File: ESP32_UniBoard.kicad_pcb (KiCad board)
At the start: 2 copper layers, 32 x 43.8 mm, 32 parts, among them J1 USB_C_Receptacle_USB2.0, J2 Conn_01x06_Socket, J3 Hirose DF40C, SW1 SW_Push, SW2 SW_Push, U1 ESP32-S3-WROOM-1, U2 SPX3819M5-L-3-3, U3 USBLC6-2SC6

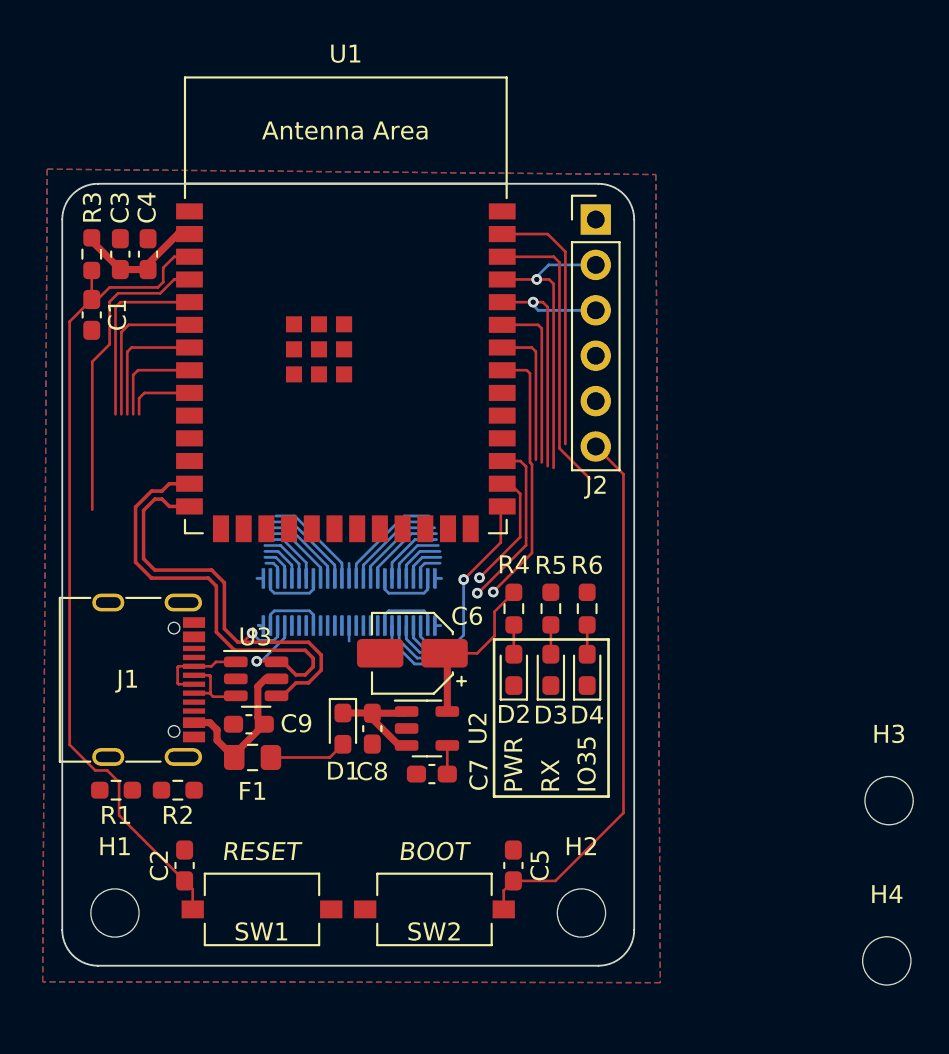
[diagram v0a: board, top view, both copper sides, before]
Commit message: PCB rework
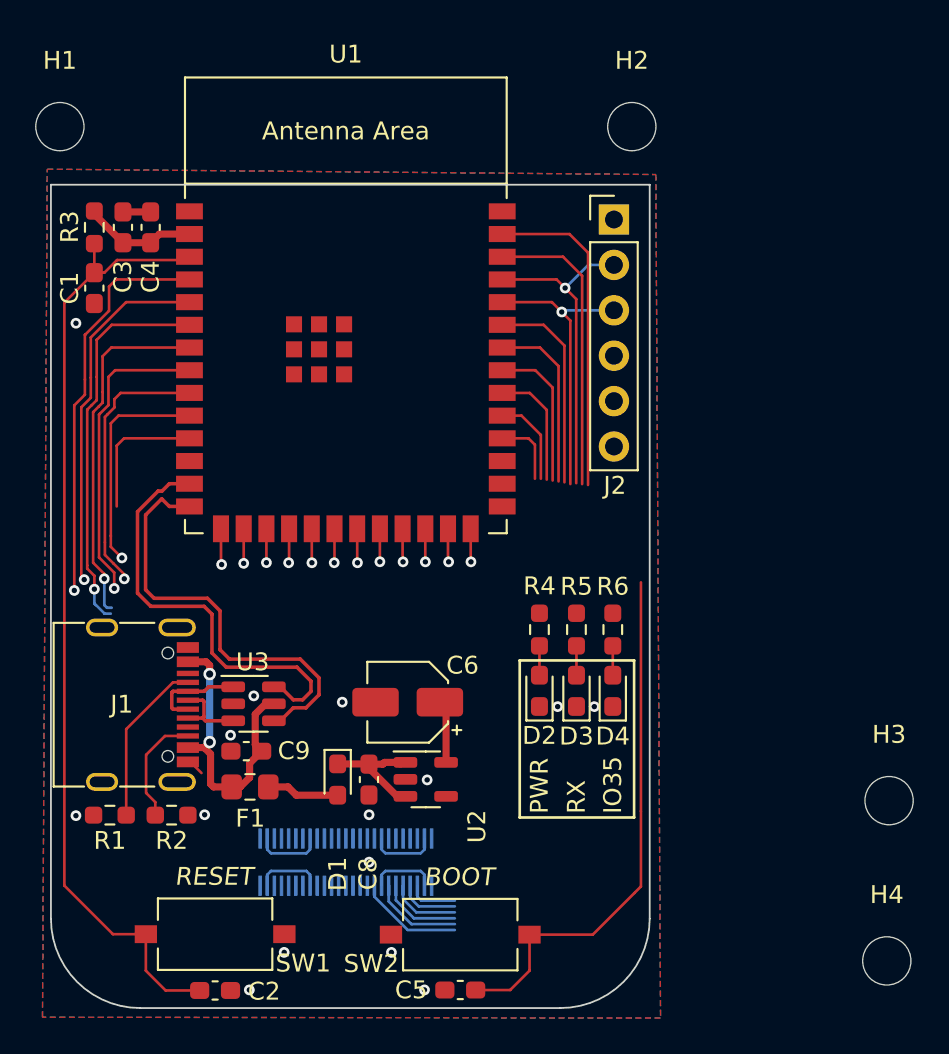
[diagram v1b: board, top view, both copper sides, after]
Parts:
- removed C7: 100nF, Capacitor_SMD:C_0603_1608Metric_Pad1.08x0.95mm_HandSolder
- moved H1 44.1 mm to (105.1, 47.3)
- moved H2 44.1 mm to (137.1, 47.3)
- moved J3 14.6 mm to (121.1, 88.5)
- moved C5 7.58 mm to (127.5, 95.6), turned to 0 degrees
- moved C2 7.20 mm to (113.8, 95.6), turned to 180 degrees
- moved SW1 2.97 mm to (113.8, 92.5)
- moved D1 2.86 mm to (120.7, 83.8)
- moved C8 2.85 mm to (122.4, 83.8)
- moved U2 2.85 mm to (125.6, 83.8)
- moved C6 2.75 mm to (124.6, 79.5)
- moved SW2 2.02 mm to (127.5, 92.5)
- moved D2 1.85 mm to (131.9, 78.9)
- moved D3 1.85 mm to (134.0, 78.9)
- moved D4 1.85 mm to (136.1, 78.9)
- moved R4 1.85 mm to (131.9, 75.4)
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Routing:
- net /BOOT: track 44.2 -> 34.4 mm, vias 1 -> 0
- net /GPIO17: track 2.58 -> 12.4 mm, vias 0 -> 1
- net Net-(J1-CC1): track 0.00 -> 9.35 mm
- net /GPIO40: track 17.8 -> 8.42 mm, vias 1 -> 0
- net /GPIO36: track 12.0 -> 3.38 mm, vias 1 -> 0
- net /GPIO6: track 13.3 -> 21.8 mm, vias 0 -> 1
- net /GPIO7: track 11.6 -> 19.9 mm, vias 0 -> 1
- net /GPIO16: track 6.99 -> 15.1 mm, vias 0 -> 1
- net /GPIO15: track 9.19 -> 17.1 mm, vias 0 -> 1
- net /GPIO48: track 0.00 -> 7.75 mm, vias 0 -> 1
- net VBUS: track 9.44 -> 16.9 mm, vias 0 -> 2
- net +3V3: track 24.5 -> 17.5 mm
- net /EN: track 46.4 -> 53.5 mm
- net Net-(J1-CC2): track 0.00 -> 6.36 mm
- net /GPIO35: track 9.72 -> 3.95 mm, vias 1 -> 0
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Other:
- board size 32 x 43.8 mm -> 33.5 x 46.1 mm
